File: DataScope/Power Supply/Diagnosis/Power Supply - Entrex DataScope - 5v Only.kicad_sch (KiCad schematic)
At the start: 41 parts, among them Q1 MPS3638, Q2 PN3569, Q3 PN3569, Q4 PS3638, Q5 2N4918, Q6 2N3055, Q7 PN3569

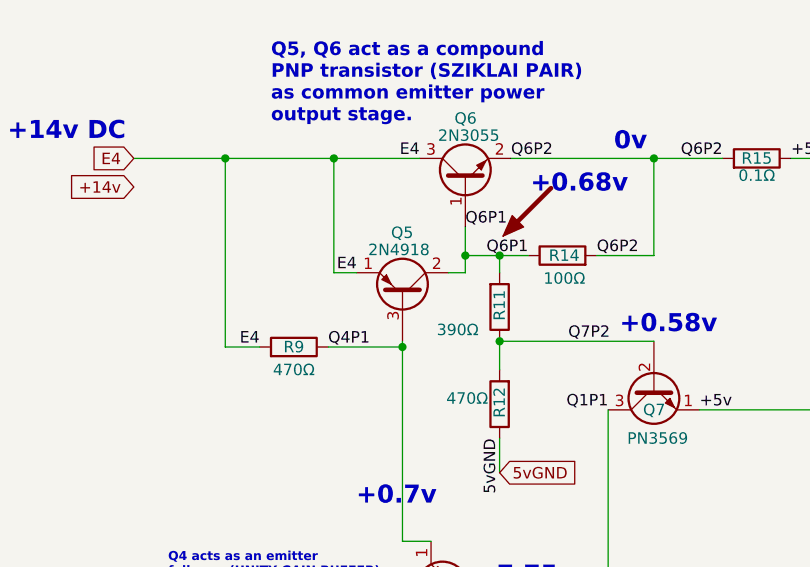
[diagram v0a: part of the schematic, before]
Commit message: junk
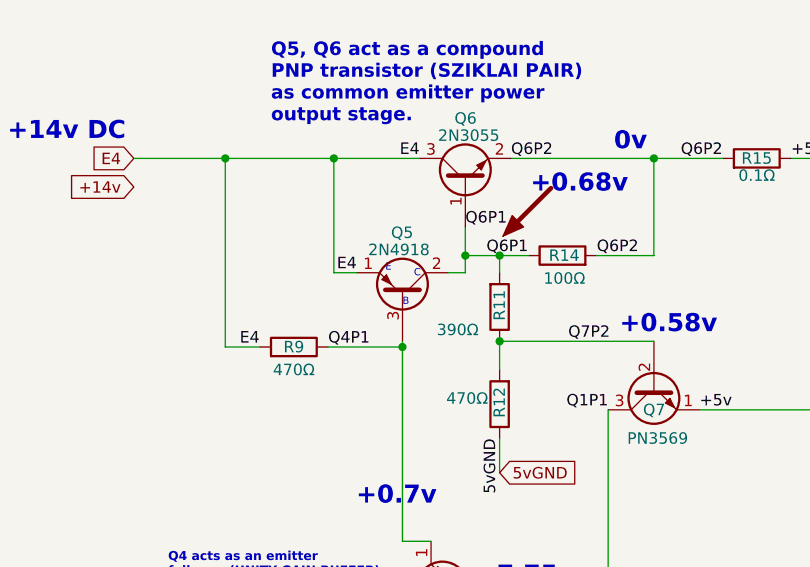
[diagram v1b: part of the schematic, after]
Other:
- note added: "B"
- note added: "C"
- note added: "E"
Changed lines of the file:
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@@
     (effects (font (size 3 3) (thickness 0.6) bold) (justify left bottom))
+  )
+  (text "C" (at 122.555 59.69 0)
+    (effects (font (size 0.8 0.8)) (justify left bottom))
   )
   (text "v AC" (at 29.845 107.823 0)
@@
   (text "0v" (at 180.975 45.72 0)
     (effects (font (size 2 2) (thickness 0.4) bold (color 255 2 13 1)) (justify left bottom))
+  )
+  (text "B\n" (at 121.285 62.865 0)
+    (effects (font (size 0.8 0.8)) (justify left bottom))
   )
   (text "R18, C4 provide damping at\nthe output." (at 288.29 65.405 0)
@@
     (effects (font (size 2 2) (thickness 0.4) bold) (justify left bottom))
   )
+  (text "E" (at 119.38 59.055 0)
+    (effects (font (size 0.8 0.8)) (justify left bottom))
+  )
   (label "C1+" (at 50.419 121.285 0) (fields_autoplaced)

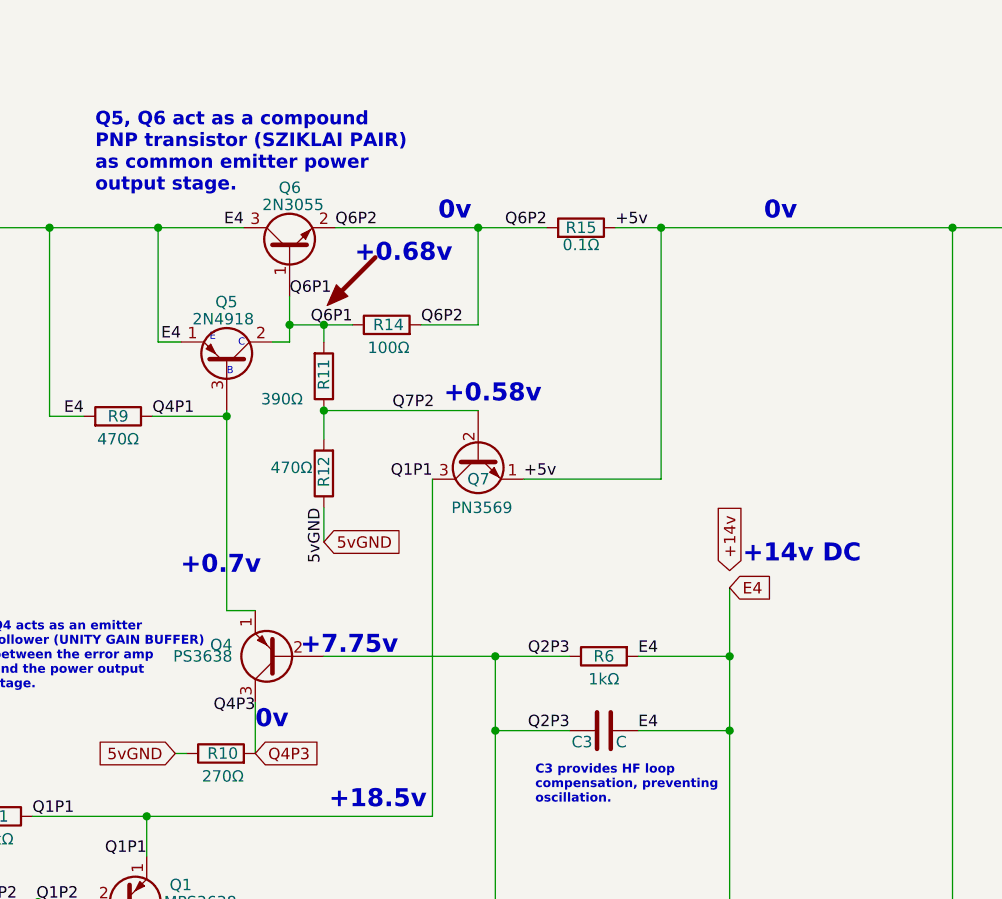
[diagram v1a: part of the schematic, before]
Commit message: yes
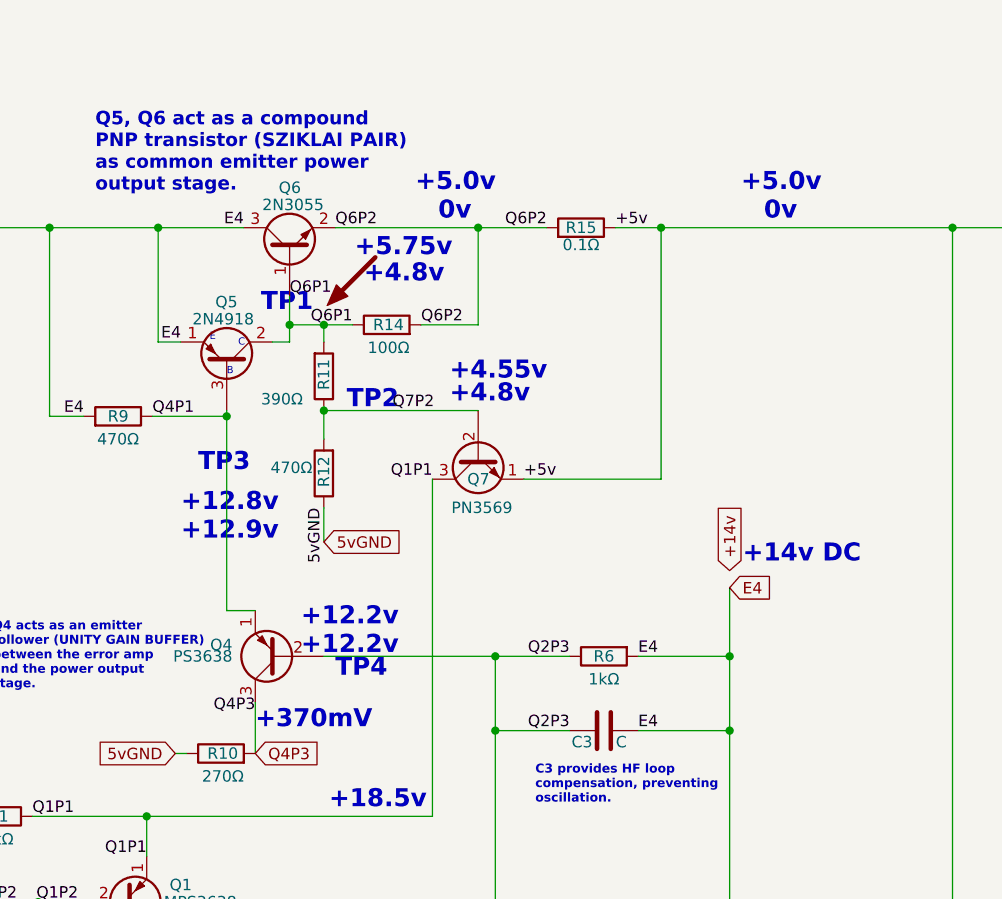
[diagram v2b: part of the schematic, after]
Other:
- note added: "+12.2v"
- note added: "+12.8v"
- note added: "+12.9v"
- note added: "+370mV"
- note added: "+4.55v"
- note added: "+4.8v"
- note added: "+5.0v"
- note added: "+5.75v"
- note added: "TP1"
- note added: "TP2"
- note added: "TP3"
- note added: "TP4"
- note removed: "+0.58v"
- note removed: "+0.68v"
- note removed: "+0.7v"
- note removed: "+7.75v"
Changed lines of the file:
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@@
     (effects (font (size 2 2) (thickness 0.4) bold) (justify left bottom))
   )
-  (text "+0.58v" (at 145.415 66.04 0)
-    (effects (font (size 2 2) (thickness 0.4) bold) (justify left bottom))
-  )
-  (text "0v" (at 124.46 102.235 0)
-    (effects (font (size 2 2) (thickness 0.4) bold (color 255 2 13 1)) (justify left bottom))
+  (text "+370mV" (at 124.46 102.235 0)
+    (effects (font (size 2 2) (thickness 0.4) bold (color 5 119 14 1)) (justify left bottom))
   )
   (text "Q1, Q7, CR5, R15, R11, R12 \nprovide output current \nlimiting."
@@
     (effects (font (size 2 2) (thickness 0.4) bold) (justify left bottom))
   )
-  (text "+0.68v" (at 135.509 50.419 0)
-    (effects (font (size 2 2) (thickness 0.4) bold) (justify left bottom))
+  (text "+5.75v" (at 135.509 49.784 0)
+    (effects (font (size 2 2) (thickness 0.4) bold (color 5 134 17 1)) (justify left bottom))
   )
   (text "0v" (at 180.975 45.72 0)
@@
     (effects (font (size 0.8 0.8)) (justify left bottom))
   )
+  (text "TP2" (at 134.62 66.675 0)
+    (effects (font (size 2 2) (thickness 0.4) bold (color 113 4 103 1)) (justify left bottom))
+  )
+  (text "+4.55v" (at 146.05 63.5 0)
+    (effects (font (size 2 2) (thickness 0.4) bold (color 5 134 17 1)) (justify left bottom))
+  )
   (text "R18, C4 provide damping at\nthe output." (at 288.29 65.405 0)
     (effects (font (size 2 2) (thickness 0.6) bold) (justify left bottom))
@@
     (effects (font (size 2 2) (thickness 0.4) bold) (justify left bottom))
   )
-  (text "+7.75v" (at 140.335 93.98 0)
-    (effects (font (size 2 2) (thickness 0.4) bold) (justify right bottom))
+  (text "+12.2v" (at 129.54 90.805 0)
+    (effects (font (size 2 2) (thickness 0.4) bold (color 5 134 17 1)) (justify left bottom))
+  )
+  (text "+12.2v" (at 129.54 93.98 0)
+    (effects (font (size 2 2) (thickness 0.4) bold (color 255 0 24 1)) (justify left bottom))
+  )
+  (text "+4.8v" (at 136.525 52.705 0)
+    (effects (font (size 2 2) (thickness 0.4) bold (color 255 0 24 1)) (justify left bottom))
+  )
+  (text "+5.0v" (at 142.24 42.545 0)
+    (effects (font (size 2 2) (thickness 0.4) bold (color 5 134 17 1)) (justify left bottom))
+  )
+  (text "+4.8v" (at 146.05 66.04 0)
+    (effects (font (size 2 2) (thickness 0.4) bold (color 255 0 24 1)) (justify left bottom))
   )
   (text "+3.3v" (at 160.02 143.51 0)
@@
   (text "+14v DC" (at 61.214 91.948 0)
     (effects (font (size 2 2) (thickness 0.4) bold) (justify right bottom))
+  )
+  (text "TP3" (at 118.11 73.66 0)
+    (effects (font (size 2 2) (thickness 0.4) bold (color 113 4 103 1)) (justify left bottom))
+  )
+  (text "+12.8v" (at 116.205 78.105 0)
+    (effects (font (size 2 2) (thickness 0.4) bold (color 5 134 17 1)) (justify left bottom))
+  )
+  (text "+5.0v" (at 178.435 42.545 0)
+    (effects (font (size 2 2) (thickness 0.4) bold (color 5 134 17 1)) (justify left bottom))
   )
   (text "R13, R8, R5, R14 set the\noutput voltage.\n" (at 194.945 144.78 0)
@@
     (effects (font (size 1.5 1.5) (thickness 0.6) bold) (justify left bottom))
   )
+  (text "TP4\n" (at 133.35 96.52 0)
+    (effects (font (size 2 2) (thickness 0.4) bold (color 113 4 103 1)) (justify left bottom))
+  )
   (text "+18.5v" (at 143.51 111.125 0)
     (effects (font (size 2 2) (thickness 0.4) bold) (justify right bottom))
+  )
+  (text "TP1" (at 125.095 55.88 0)
+    (effects (font (size 2 2) (thickness 0.4) bold (color 113 4 103 1)) (justify left bottom))
   )
   (text "Q2, Q3 act as a differential\npair error amplifier, comparing\nthe 5v output with a reference\nvoltage developed by CR6."
@@
     (effects (font (size 1 1) (thickness 0.6) bold) (justify left bottom))
   )
-  (text "+0.7v" (at 125.095 85.09 0)
-    (effects (font (size 2 2) (thickness 0.4) bold) (justify right bottom))
+  (text "+12.9v" (at 116.205 81.28 0)
+    (effects (font (size 2 2) (thickness 0.4) bold (color 255 0 24 1)) (justify left bottom))
   )
   (text "+23v DC" (at 56.007 124.46 0)

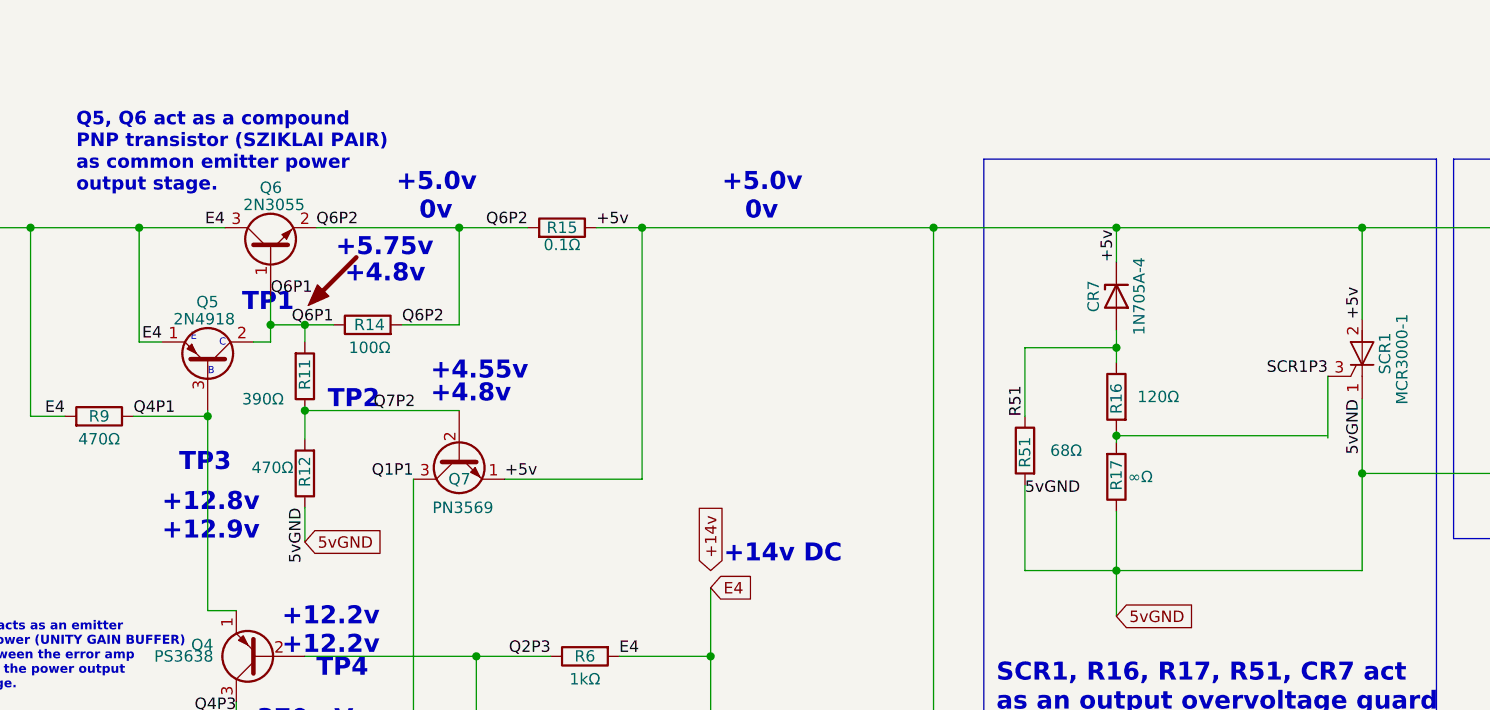
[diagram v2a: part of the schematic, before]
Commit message: fix?
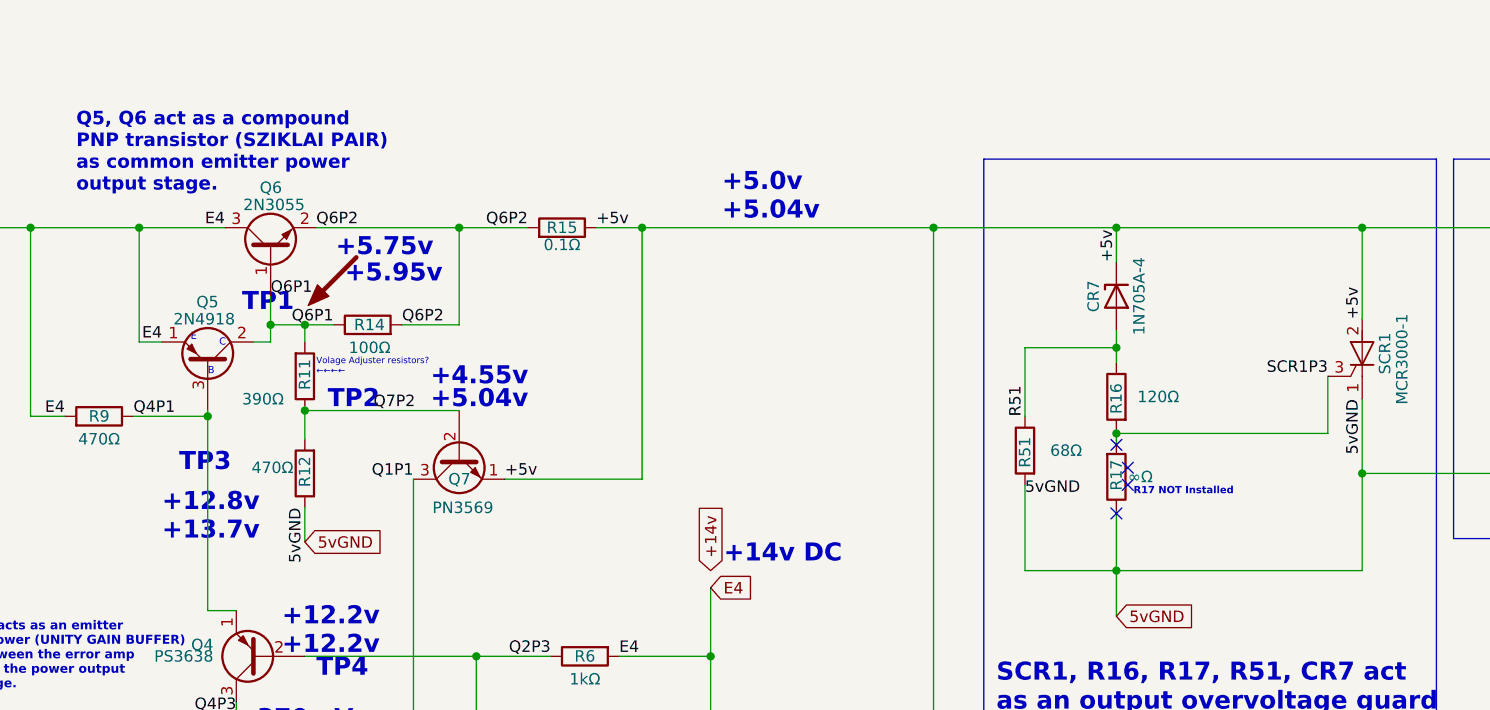
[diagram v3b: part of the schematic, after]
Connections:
- net SCR1P3: now also R16.2, R17.2
- no-connect marks 0 -> 4
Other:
- note added: "+13.7v"
- note added: "+5.04v"
- note added: "+5.95v"
- note added: "R17 NOT Installed"
- note added: "Volage Adjuster resistors? ←←←←"
- note removed: "+12.9v"
- note removed: "+4.8v"
- note removed: "0v"
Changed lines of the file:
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@@
   (junction (at 222.25 59.69) (diameter 0) (color 0 0 0 0)
   )
-  (junction (at 222.25 69.469) (diameter 0) (color 0 0 0 0)
-  )
   (junction (at 164.465 168.275) (diameter 0) (color 0 0 0 0)
   )
@@
   (junction (at 132.08 66.675) (diameter 0) (color 0 0 0 0)
   )
+  (junction (at 222.25 69.215) (diameter 0) (color 0 0 0 0)
+  )
   (junction (at 151.13 93.98) (diameter 0) (color 0 0 0 0)
   )
@@
   (junction (at 42.799 128.905) (diameter 0) (color 0 0 0 0)
   )
+  (no_connect (at 222.25 78.105))
+  (no_connect (at 223.52 74.93))
+  (no_connect (at 223.52 73.025))
+  (no_connect (at 222.25 70.485))
   (wire (pts (xy 121.285 67.31) (xy 121.285 88.9))
     (stroke (width 0) (type default))
@@
     (stroke (width 0) (type default))
   )
-  (wire (pts (xy 245.618 69.469) (xy 222.25 69.469))
-    (stroke (width 0) (type default))
-  )
   (wire (pts (xy 112.395 111.76) (xy 144.145 111.76))
     (stroke (width 0) (type default))
@@
     (stroke (width 0) (type default))
   )
-  (wire (pts (xy 222.25 68.961) (xy 222.25 69.469))
+  (wire (pts (xy 222.25 68.961) (xy 222.25 69.215))
     (stroke (width 0) (type default))
   )
@@
     (stroke (width 0) (type default))
   )
-  (wire (pts (xy 222.25 69.469) (xy 222.25 70.231))
-    (stroke (width 0) (type default))
-  )
-  (wire (pts (xy 245.745 62.865) (xy 245.745 69.723))
-    (stroke (width 0) (type default))
-  )
   (wire (pts (xy 222.25 84.455) (xy 222.25 89.535))
     (stroke (width 0) (type default))
@@
     (stroke (width 0) (type default))
   )
+  (wire (pts (xy 222.25 69.215) (xy 222.25 70.231))
+    (stroke (width 0) (type default))
+  )
   (wire (pts (xy 112.395 136.525) (xy 116.205 136.525))
     (stroke (width 0) (type default))
@@
     (stroke (width 0) (type default))
   )
+  (wire (pts (xy 245.745 69.215) (xy 222.25 69.215))
+    (stroke (width 0) (type default))
+  )
   (wire (pts (xy 212.09 59.69) (xy 222.25 59.69))
     (stroke (width 0) (type default))
@@
   )
   (wire (pts (xy 132.08 57.15) (xy 132.08 59.055))
+    (stroke (width 0) (type default))
+  )
+  (wire (pts (xy 245.745 62.865) (xy 245.745 69.215))
     (stroke (width 0) (type default))
   )
@@
     (effects (font (size 2 2) (thickness 0.4) bold (color 5 134 17 1)) (justify left bottom))
   )
-  (text "0v" (at 180.975 45.72 0)
+  (text "+5.04v" (at 178.435 45.72 0)
     (effects (font (size 2 2) (thickness 0.4) bold (color 255 2 13 1)) (justify left bottom))
   )
@@
     (effects (font (size 2 2) (thickness 0.4) bold (color 113 4 103 1)) (justify left bottom))
   )
-  (text "+4.55v" (at 146.05 63.5 0)
+  (text "+4.55v" (at 146.05 64.135 0)
     (effects (font (size 2 2) (thickness 0.4) bold (color 5 134 17 1)) (justify left bottom))
   )
@@
     (effects (font (size 2 2) (thickness 0.4) bold (color 255 0 24 1)) (justify left bottom))
   )
-  (text "+4.8v" (at 136.525 52.705 0)
+  (text "+5.95v" (at 136.525 52.705 0)
     (effects (font (size 2 2) (thickness 0.4) bold (color 255 0 24 1)) (justify left bottom))
   )
-  (text "+5.0v" (at 142.24 42.545 0)
-    (effects (font (size 2 2) (thickness 0.4) bold (color 5 134 17 1)) (justify left bottom))
-  )
-  (text "+4.8v" (at 146.05 66.04 0)
+  (text "+5.04v" (at 146.05 66.675 0)
     (effects (font (size 2 2) (thickness 0.4) bold (color 255 0 24 1)) (justify left bottom))
   )
@@
     (effects (font (size 2 2) (thickness 0.6) bold) (justify left bottom))
   )
-  (text "0v" (at 144.78 45.72 0)
-    (effects (font (size 2 2) (thickness 0.4) bold (color 255 2 13 1)) (justify left bottom))
-  )
   (text "+14v DC" (at 191.77 83.82 0)
     (effects (font (size 2 2) (thickness 0.4) bold) (justify right bottom))
@@
     (effects (font (size 2 2) (thickness 0.4) bold) (justify right bottom))
   )
+  (text "R17 NOT Installed\n" (at 224.155 76.2 0)
+    (effects (font (size 0.8 0.8) (thickness 0.16) bold (color 255 0 19 1)) (justify left bottom))
+  )
   (text "Addtional Pictures found at\nhttps://github.com/ForgottenMachines/Entrex/tree/main/DataScope/Power%20Supply/Images\n"
     (at 16.51 20.955 0)
@@
     (effects (font (size 2 2) (thickness 0.4) bold) (justify right bottom))
   )
+  (text "Volage Adjuster resistors?\n←←←← " (at 133.35 62.865 0)
+    (effects (font (size 0.7 0.7)) (justify left bottom))
+  )
   (text "C3 provides HF loop \ncompensation, preventing\noscillation."
     (at 155.575 110.49 0)
     (effects (font (size 1 1) (thickness 0.6) bold) (justify left bottom))
   )
-  (text "+12.9v" (at 116.205 81.28 0)
+  (text "+13.7v" (at 116.205 81.28 0)
     (effects (font (size 2 2) (thickness 0.4) bold (color 255 0 24 1)) (justify left bottom))
   )
